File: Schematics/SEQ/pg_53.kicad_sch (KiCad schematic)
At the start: 6 parts, among them U5401 F30, U5402 F148, U5403 F02, U5404 F20, U5405 F240, U5406 F374

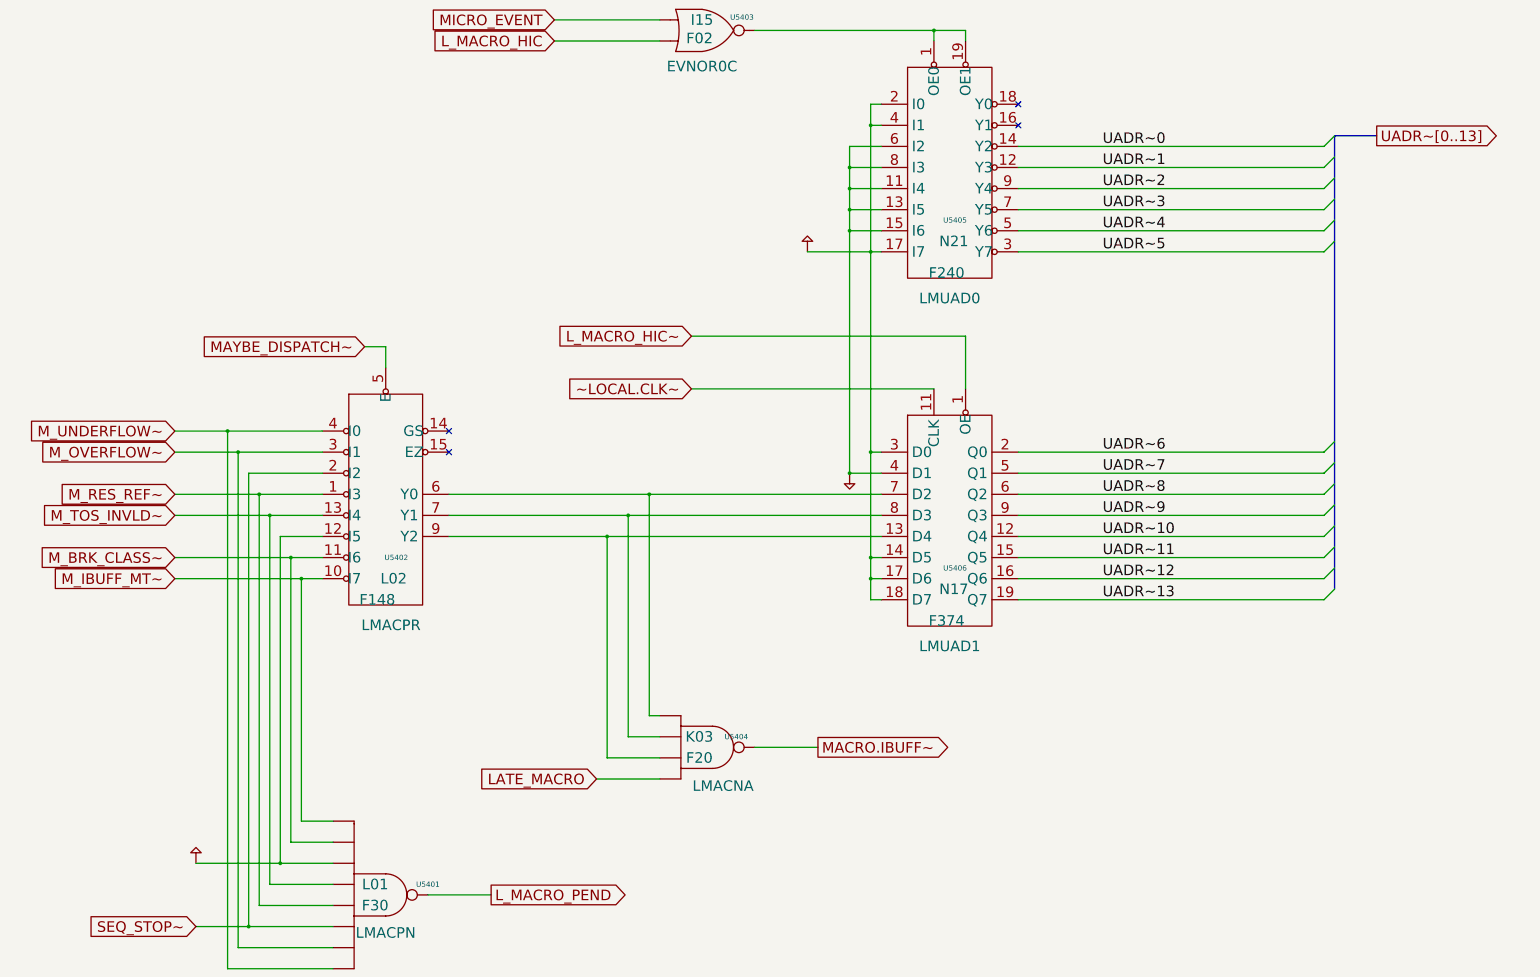
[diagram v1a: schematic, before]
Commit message: Megacompification
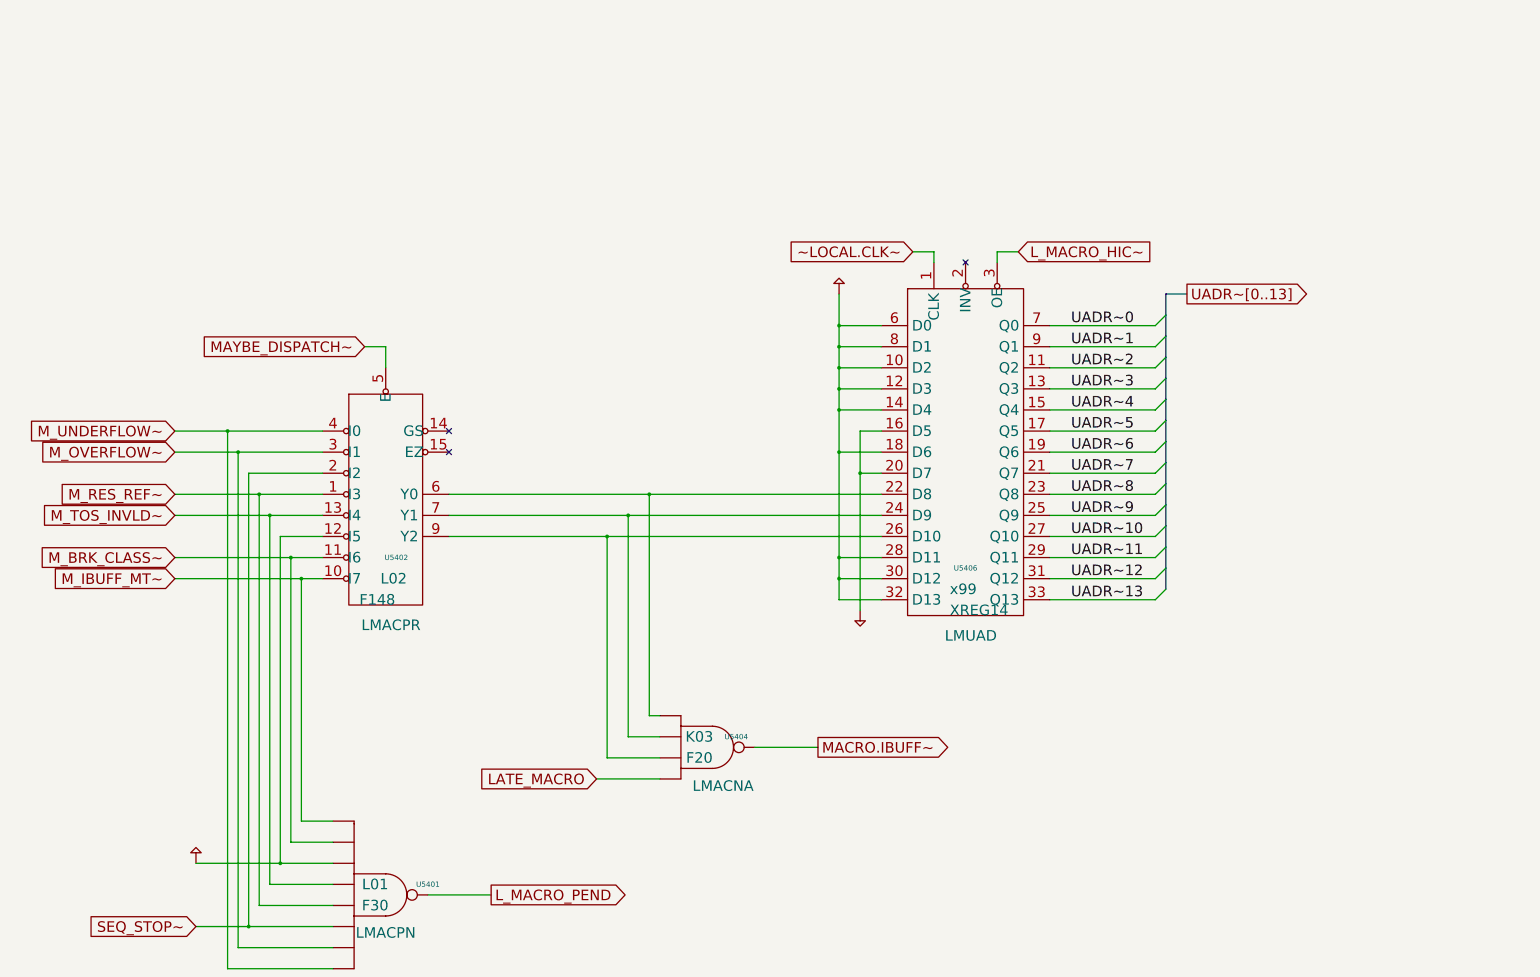
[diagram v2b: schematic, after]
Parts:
- removed U5403: F02, symbol r1000:F02
- removed U5405: F240, symbol r1000:F240
- U5406: value F374 -> XREG14; symbol r1000:F374 -> r1000:XREG14; Location N17 -> x99; Name LMUAD1 -> LMUAD
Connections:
- net L_MACRO_HIC~: now also U5406.3 (OE); no longer U5406.1 (OE)
- net PD: now also U5406.16 (D5), U5406.20 (D7); no longer U5406.4 (D1)
- net PU: now also U5406.10 (D2), U5406.12 (D3), U5406.28 (D11), U5406.30 (D12), U5406.32 (D13), U5406.6 (D0), U5406.8 (D1); no longer U5406.17 (D6), U5406.3 (D0)
- net UADR~0: now also U5406.7 (Q0)
- net UADR~1: now also U5406.9 (Q1)
- net UADR~10: now also U5406.27 (Q10); no longer U5406.12 (Q4)
- net UADR~11: now also U5406.29 (Q11); no longer U5406.15 (Q5)
- net UADR~12: now also U5406.31 (Q12); no longer U5406.16 (Q6)
- net UADR~13: now also U5406.33 (Q13); no longer U5406.19 (Q7)
- net UADR~2: now also U5406.11 (Q2)
- net UADR~3: now also U5406.13 (Q3)
- net UADR~4: now also U5406.15 (Q4)
- net UADR~5: now also U5406.17 (Q5)
- net UADR~6: now also U5406.19 (Q6); no longer U5406.2 (Q0)
- net UADR~7: now also U5406.21 (Q7); no longer U5406.5 (Q1)
- net UADR~8: now also U5406.23 (Q8); no longer U5406.6 (Q2)
- net UADR~9: now also U5406.25 (Q9); no longer U5406.9 (Q3)
- net ~LOCAL.CLK~: now also U5406.1 (CLK); no longer U5406.11 (CLK)
- net at U5402.6 (Y0), U5404.1 (D0): now also U5406.22 (D8); no longer U5406.7 (D2)
- net at U5402.7 (Y1), U5404.2 (D1): now also U5406.24 (D9); no longer U5406.8 (D3)
- net at U5402.9 (Y2), U5404.4 (D2): now also U5406.26 (D10); no longer U5406.13 (D4)
- no-connect marks 4 -> 3
